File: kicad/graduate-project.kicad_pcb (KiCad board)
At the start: 2 copper layers, 43.2 x 76.2 mm, 16 parts, among them J1 Power, J2 GY-9250, J3 HM-10, J4 Left Motor, J5 Right Motor, U1 NUCLEO-L432KC, U2 DRV8847PWP

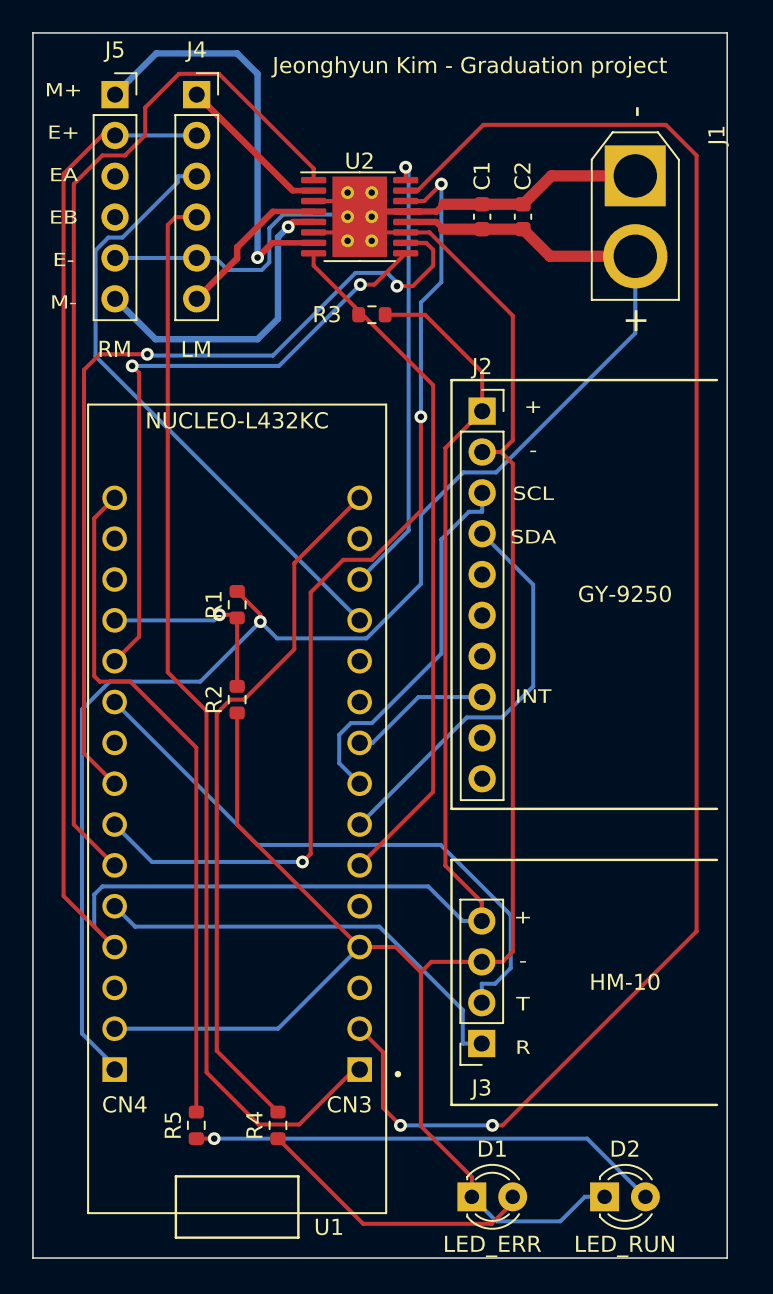
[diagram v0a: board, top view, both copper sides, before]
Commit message: Update pdf plots
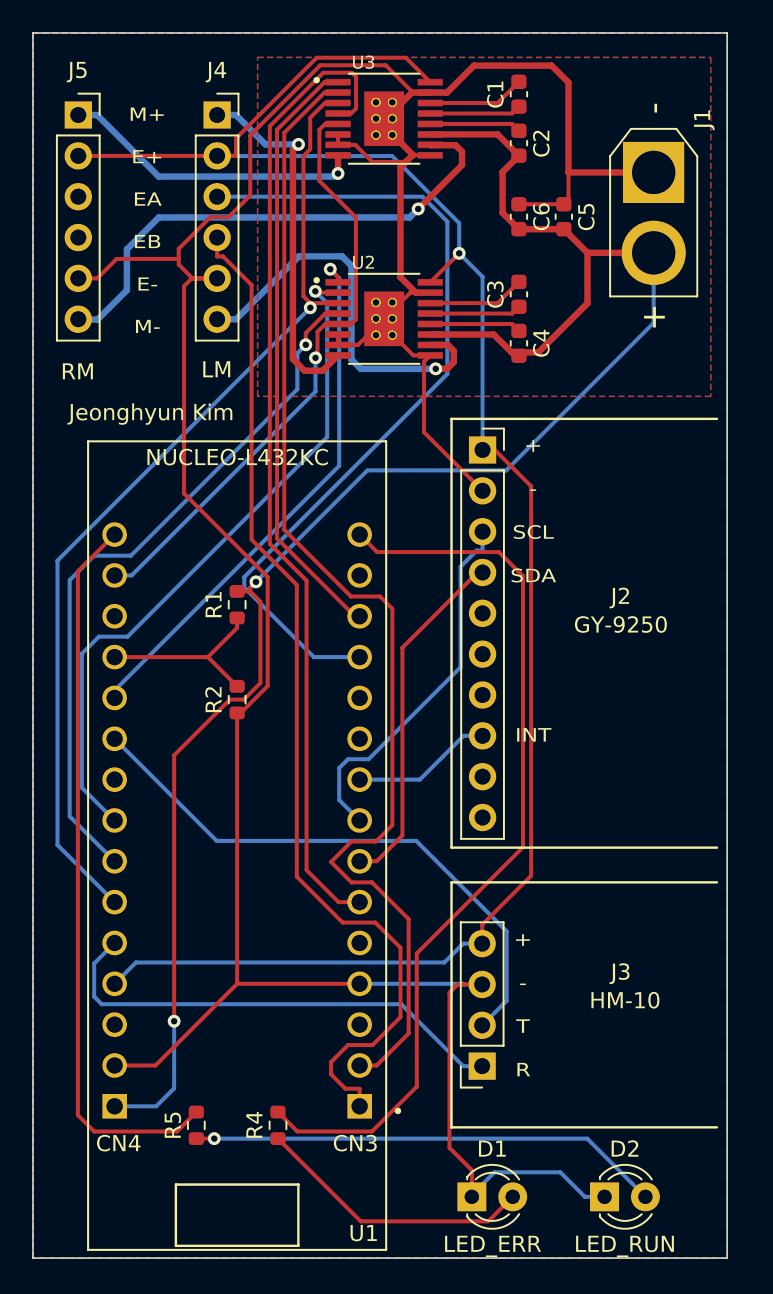
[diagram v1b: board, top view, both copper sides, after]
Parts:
- removed R3: 10k, Resistor_SMD:R_0603_1608Metric
- added ?: , , F.Cu at (72.1, 55.9)
- added ?: , , F.Cu at (72.1, 42.4)
- added ?: , , F.Cu at (73.2, 55.9)
- added ?: , , F.Cu at (72.1, 56.9)
- added ?: , , F.Cu at (73.2, 56.9)
- added ?: , , F.Cu at (72.1, 44.5)
- added ?: , , F.Cu at (73.2, 44.5)
- added ?: , , F.Cu at (72.1, 43.4)
- added ?: , , F.Cu at (73.2, 42.4)
- added ?: , , F.Cu at (72.1, 54.9)
- added ?: , , F.Cu at (73.2, 54.9)
- added ?: , , F.Cu at (73.2, 43.4)
- added C3: 22n, Capacitor_SMD:C_0603_1608Metric, F.Cu at (81.0, 54.4)
- added C4: 100n, Capacitor_SMD:C_0603_1608Metric, F.Cu at (81.0, 57.4)
- added C5: 10u, Capacitor_SMD:C_0603_1608Metric, F.Cu at (83.8, 49.5)
- added C6: 0.1u, Capacitor_SMD:C_0603_1608Metric, F.Cu at (81.0, 49.5)
- added U3: DRV8874PWPR, DRV8874PWPR:SOP65P640X120-17N, F.Cu at (72.6, 43.4)
- C1: value 10u -> 22n
- C2: value 0.1u -> 100n
- U2: value DRV8847PWP -> DRV8874PWPR; footprint Package_SO:HTSSOP-16-1EP_4.4x5mm_P0.65mm_EP3.4x5mm_Mask2.46x2.31mm_ThermalVias -> DRV8874PWPR:SOP65P640X120-17N
- moved C1 7.96 mm to (81.0, 41.9)
- moved U2 6.53 mm to (72.6, 55.9)
- moved C2 4.58 mm to (81.0, 45.0), turned to -90 degrees
- moved J5 2.62 mm to (53.6, 43.2)
- moved J2 2.41 mm to (78.8, 64.0)
- moved U1 2.29 mm to (63.5, 88.6)
- moved J4 1.80 mm to (62.3, 43.2)
- moved J3 1.41 mm to (78.7, 102.4)
- moved J1 1.16 mm to (89.4, 46.8)
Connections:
- C1 pad 1: BATT_VIN -> Net-(C1-Pad1)
- C1 pad 2: BATT_GND -> Net-(C1-Pad2)
- C2 pad 1: BATT_VIN -> Net-(C2-Pad1)
- C2 pad 2: BATT_GND -> BATT_VIN
- J4 pad 1: Net-(J4-Pad1) -> Net-(U2-Pad8)
- J4 pad 6: Net-(J4-Pad6) -> Net-(U2-Pad10)
- U1 pad CN3_6: M_FAULT -> M_FAULT1
- U1 pad CN4_14: unconnected-(U1-PadCN4_14) -> 3_3V
- U1 pad CN4_7: M_MODE -> M_FAULT2
- U2 pad 1: M_OFF -> M_IN3
- U2 pad 10: M_IN4 -> Net-(U2-Pad10)
- U2 pad 11: BATT_GND -> BATT_VIN
- U2 pad 12: BATT_VIN -> Net-(C4-Pad1)
- U2 pad 13: BATT_GND -> Net-(C3-Pad1)
- U2 pad 14: M_MODE -> Net-(C3-Pad2)
- U2 pad 15: M_IN2 -> BATT_GND
- U2 pad 16: M_IN1 -> ENC_VCC
- U2 pad 2: Net-(J4-Pad1) -> M_IN4
- U2 pad 3: BATT_GND -> M_OFF
- U2 pad 4: Net-(J4-Pad6) -> M_FAULT2
- U2 pad 5: Net-(J5-Pad6) -> 3_3V
- U2 pad 7: Net-(J5-Pad1) -> BATT_GND
- U2 pad 8: M_FAULT -> Net-(U2-Pad8)
- U2 pad 9: M_IN3 -> BATT_GND
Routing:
- net M_MODE: track 62.1 -> 0.00 mm, vias 3 -> 0
- net M_FAULT1: track 0.00 -> 61.4 mm
- net M_FAULT2: track 0.00 -> 43.9 mm, vias 0 -> 1
- net M_FAULT: track 43.0 -> 0.00 mm
- net 3_3V: track 0.00 -> 37.8 mm, vias 0 -> 1
- net BATT_GND: track 172.1 -> 203.1 mm
- net M_IN2: track 99.3 -> 73.3 mm, vias 2 -> 0
- net Net-(U2-Pad10): track 0.00 -> 25.1 mm, vias 0 -> 1
- net Net-(U2-Pad8): track 0.00 -> 22.8 mm, vias 0 -> 1
- net BATT_VIN: track 93.2 -> 110.7 mm, vias 1 -> 2
- net ENC_1A: track 38.2 -> 51.9 mm
- net ENC_VCC: track 131.0 -> 117.3 mm, vias 0 -> 1
- net Net-(J5-Pad6): track 19.4 -> 32.3 mm
- net LED_ERR: track 44.0 -> 56.0 mm
- net M_IN4: track 54.7 -> 42.9 mm, vias 2 -> 1
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- added copper zone on B.Cu, net BATT_GND
- added copper zone on F.Cu, net BATT_GND
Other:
- board text added: "Jeonghyun Kim"
- board text removed: "Jeonghyun Kim - Graduation project"
